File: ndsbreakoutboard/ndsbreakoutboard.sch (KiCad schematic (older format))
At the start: 2 parts, among them J1 Conn_01x17_Female, U1 ndsPADS

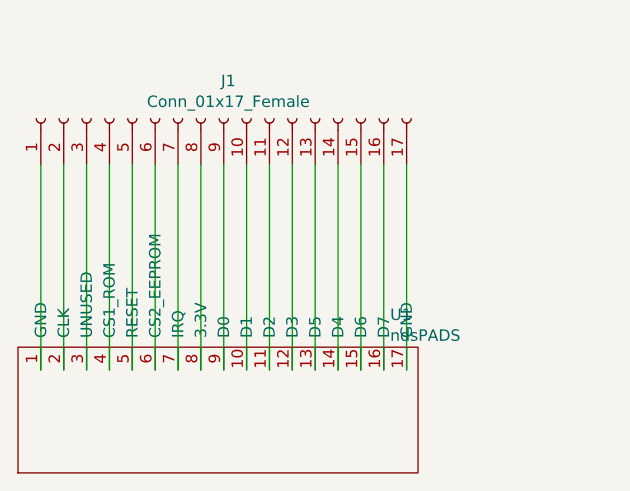
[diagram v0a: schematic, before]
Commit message: Commit before rebuilding netlist with pin headers
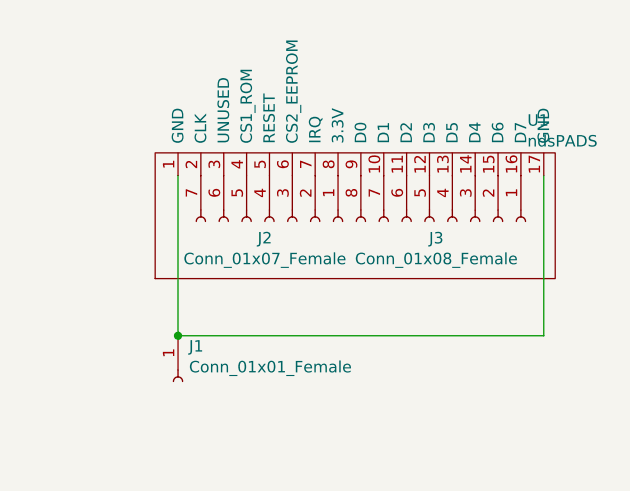
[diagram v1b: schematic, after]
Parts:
- removed J1: Conn_01x17_Female, Connector_PinHeader_2.54mm:PinHeader_1x17_P2.54mm_Vertical, symbol Connector:Conn_01x17_Female
- added J1: Conn_01x01_Female, Connector_PinHeader_1.00mm:PinHeader_1x01_P1.00mm_Horizontal, symbol Connector:Conn_01x01_Female
- added J2: Conn_01x07_Female, Connector_PinHeader_1.00mm:PinHeader_1x07_P1.00mm_Horizontal, symbol Connector:Conn_01x07_Female
- added J3: Conn_01x08_Female, Connector_PinHeader_1.00mm:PinHeader_1x08_P1.00mm_Horizontal, symbol Connector:Conn_01x08_Female
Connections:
- net at U1.1 (GND): now also U1.17 (GND), J1.1 (Pin_1)
- net at U1.10 (D1): now also J3.7 (Pin_7)
- net at U1.11 (D2): now also J3.6 (Pin_6)
- net at U1.12 (D3): now also J3.5 (Pin_5)
- net at U1.13 (D5): now also J3.4 (Pin_4)
- net at U1.14 (D4): now also J3.3 (Pin_3)
- net at U1.15 (D6): now also J3.2 (Pin_2)
- net at U1.16 (D7): now also J3.1 (Pin_1)
- net at U1.2 (CLK): now also J2.7 (Pin_7)
- net at U1.3 (UNUSED): now also J2.6 (Pin_6)
- net at U1.4 (CS1_ROM): now also J2.5 (Pin_5)
- net at U1.5 (RESET): now also J2.4 (Pin_4)
- net at U1.6 (CS2_EEPROM): now also J2.3 (Pin_3)
- net at U1.7 (IRQ): now also J2.2 (Pin_2)
- net at U1.8 (3.3V): now also J2.1 (Pin_1)
- net at U1.9 (D0): now also J3.8 (Pin_8)
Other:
- moved on the sheet: U1
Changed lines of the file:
@@
 $EndDescr
-$Comp
-L Connector:Conn_01x17_Female J1
-U 1 1 5FF23434
-P 2250 2000
-F 0 "J1" V 2415 1980 50  0000 C CNN
-F 1 "Conn_01x17_Female" V 2324 1980 50  0000 C CNN
-F 2 "Connector_PinHeader_2.54mm:PinHeader_1x17_P2.54mm_Vertical" H 2250 2000 50  0001 C CNN
-F 3 "~" H 2250 2000 50  0001 C CNN
-	1    2250 2000
-	0    -1   -1   0
-$EndComp
 $Comp
 L Connector:ndsPADS U1
 U 1 1 5FF2F120
-P 2450 3400
-F 0 "U1" H 2978 3942 50  0000 L CNN
-F 1 "ndsPADS" H 2978 3851 50  0000 L CNN
-F 2 "Connector:nds_contact_pads" H 2450 3400 50  0001 C CNN
-F 3 "" H 2450 3400 50  0001 C CNN
-	1    2450 3400
+P 3050 2550
+F 0 "U1" H 3578 3092 50  0000 L CNN
+F 1 "ndsPADS" H 3578 3001 50  0000 L CNN
+F 2 "Connector:nds_contact_pads" H 3050 2550 50  0001 C CNN
+F 3 "" H 3050 2550 50  0001 C CNN
+	1    3050 2550
 	1    0    0    -1
 $EndComp
+$Comp
+L Connector:Conn_01x08_Female J3
+U 1 1 5FF67247
+P 3250 2450
+F 0 "J3" V 3323 2380 50  0000 C CNN
+F 1 "Conn_01x08_Female" V 3414 2380 50  0000 C CNN
+F 2 "Connector_PinHeader_1.00mm:PinHeader_1x08_P1.00mm_Horizontal" H 3250 2450 50  0001 C CNN
+F 3 "~" H 3250 2450 50  0001 C CNN
+	1    3250 2450
+	0    1    1    0
+$EndComp
+$Comp
+L Connector:Conn_01x07_Female J2
+U 1 1 5FF6AEC4
+P 2450 2450
+F 0 "J2" V 2523 2430 50  0000 C CNN
+F 1 "Conn_01x07_Female" V 2614 2430 50  0000 C CNN
+F 2 "Connector_PinHeader_1.00mm:PinHeader_1x07_P1.00mm_Horizontal" H 2450 2450 50  0001 C CNN
+F 3 "~" H 2450 2450 50  0001 C CNN
+	1    2450 2450
+	0    1    1    0
+$EndComp
+$Comp
+L Connector:Conn_01x01_Female J1
+U 1 1 5FF6C91E
+P 2050 3150
+F 0 "J1" V 1896 3198 50  0000 L CNN
+F 1 "Conn_01x01_Female" V 1987 3198 50  0000 L CNN
+F 2 "Connector_PinHeader_1.00mm:PinHeader_1x01_P1.00mm_Horizontal" H 2050 3150 50  0001 C CNN
+F 3 "~" H 2050 3150 50  0001 C CNN
+	1    2050 3150
+	0    1    1    0
+$EndComp
 Wire Wire Line
-	1450 2200 1450 3100
+	2050 2950 3650 2950
 Wire Wire Line
-	1550 2200 1550 3100
+	3650 2950 3650 2250
 Wire Wire Line
-	1650 2200 1650 3100
-Wire Wire Line
-	1750 2200 1750 3100
-Wire Wire Line
-	1850 2200 1850 3100
-Wire Wire Line
-	1950 2200 1950 3100
-Wire Wire Line
-	2050 2200 2050 3100
-Wire Wire Line
-	2150 2200 2150 3100
-Wire Wire Line
-	2250 2200 2250 3100
-Wire Wire Line
-	2350 2200 2350 3100
-Wire Wire Line
-	2450 2200 2450 3100
-Wire Wire Line
-	2550 2200 2550 3100
-Wire Wire Line
-	2650 2200 2650 3100
-Wire Wire Line
-	2750 3100 2750 2200
-Wire Wire Line
-	2850 2200 2850 3100
-Wire Wire Line
-	2950 2200 2950 3100
-Wire Wire Line
-	3050 2200 3050 3100
+	2050 2950 2050 2250
+Connection ~ 2050 2950
 $EndSCHEMATC
